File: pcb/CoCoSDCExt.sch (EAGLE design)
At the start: 59 parts, among them IC1 AM29F040J, IC10 YAC512-M, IC14 TL974, IC15 TL974, IC2 XC9572XLVQG64, IC3 AS6C4008SIN, IC4 SN76489R, IC5 16MHz, IC6 16MHz, IC9 YMF262-M, X1 EXPANSION_PORT_COCO, X2 EXPANSION_PORT_COCOS

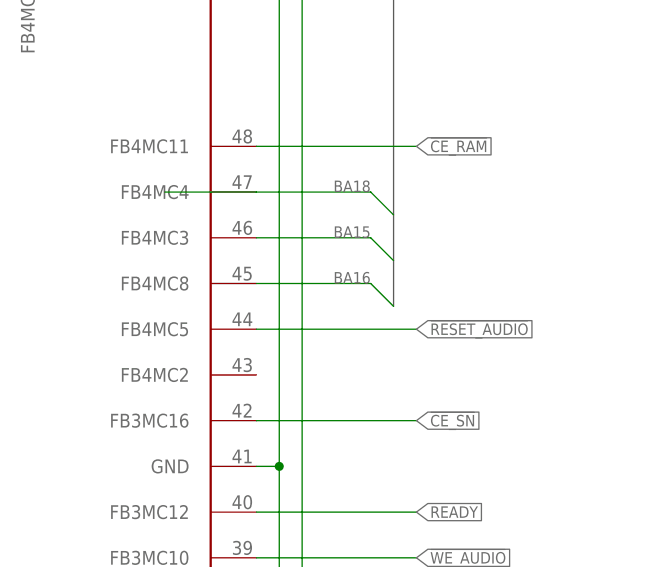
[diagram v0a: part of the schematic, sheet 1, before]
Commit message: More fixes
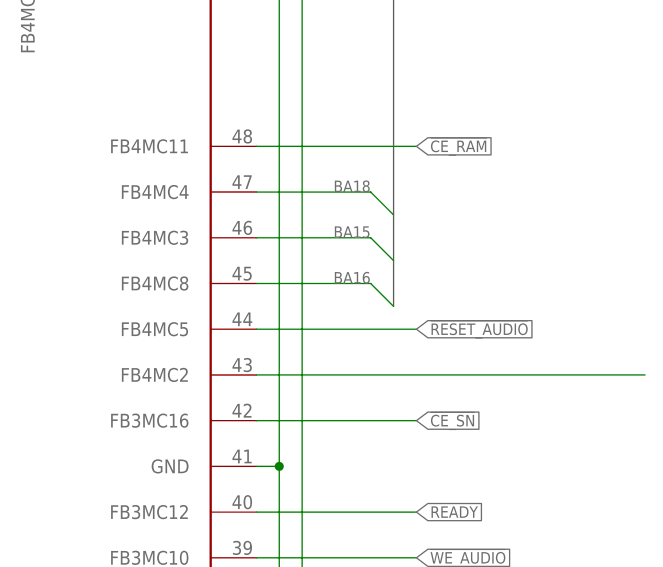
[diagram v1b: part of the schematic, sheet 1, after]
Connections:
- removed net CN_CH_0: IC4A.AUDIO
- new net N$4: IC2.FB4MC2
- net SN_CH_0: now also IC4A.AUDIO
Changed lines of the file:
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@@
 <wire x1="383.54" y1="127" x2="370.84" y2="127" width="0.1524" layer="91"/>
 <pinref part="IC2" gate="G$1" pin="FB4MC4"/>
-<wire x1="360.68" y1="127" x2="370.84" y2="127" width="0.1524" layer="91"/>
 </segment>
 </net>
@@
 <wire x1="370.84" y1="86.36" x2="388.62" y2="86.36" width="0.1524" layer="91"/>
 <label x="388.62" y="86.36" size="1.27" layer="95" xref="yes"/>
+</segment>
+</net>
+<net name="N$4" class="0">
+<segment>
+<pinref part="IC2" gate="G$1" pin="FB4MC2"/>
+<wire x1="370.84" y1="106.68" x2="414.02" y2="106.68" width="0.1524" layer="91"/>
 </segment>
 </net>
@@
 </segment>
 </net>
-<net name="CN_CH_0" class="0">
-<segment>
-<pinref part="IC4" gate="A" pin="AUDIO"/>
-<wire x1="101.6" y1="119.38" x2="104.14" y2="119.38" width="0.1524" layer="91"/>
-<label x="104.14" y="119.38" size="1.27" layer="95" xref="yes"/>
-</segment>
-</net>
 <net name="N$2" class="0">
 <segment>
@@
 <wire x1="147.32" y1="50.8" x2="144.78" y2="50.8" width="0.1524" layer="91"/>
 <label x="144.78" y="50.8" size="1.27" layer="95" rot="R180" xref="yes"/>
+</segment>
+<segment>
+<pinref part="IC4" gate="A" pin="AUDIO"/>
+<wire x1="101.6" y1="119.38" x2="104.14" y2="119.38" width="0.1524" layer="91"/>
+<label x="104.14" y="119.38" size="1.27" layer="95" xref="yes"/>
 </segment>
 </net>
@@
 </sheet>
 </sheets>
+<errors>
+</errors>
 </schematic>
 </drawing>
